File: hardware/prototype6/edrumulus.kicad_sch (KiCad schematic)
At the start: 108 parts, among them J1 Trigger Connector, J2 Raspberry Pi GPIO pins, U1 ESP32-WROOM-32U, U2 AMS1117-3.3, U3 MCP1754S-3302xMB

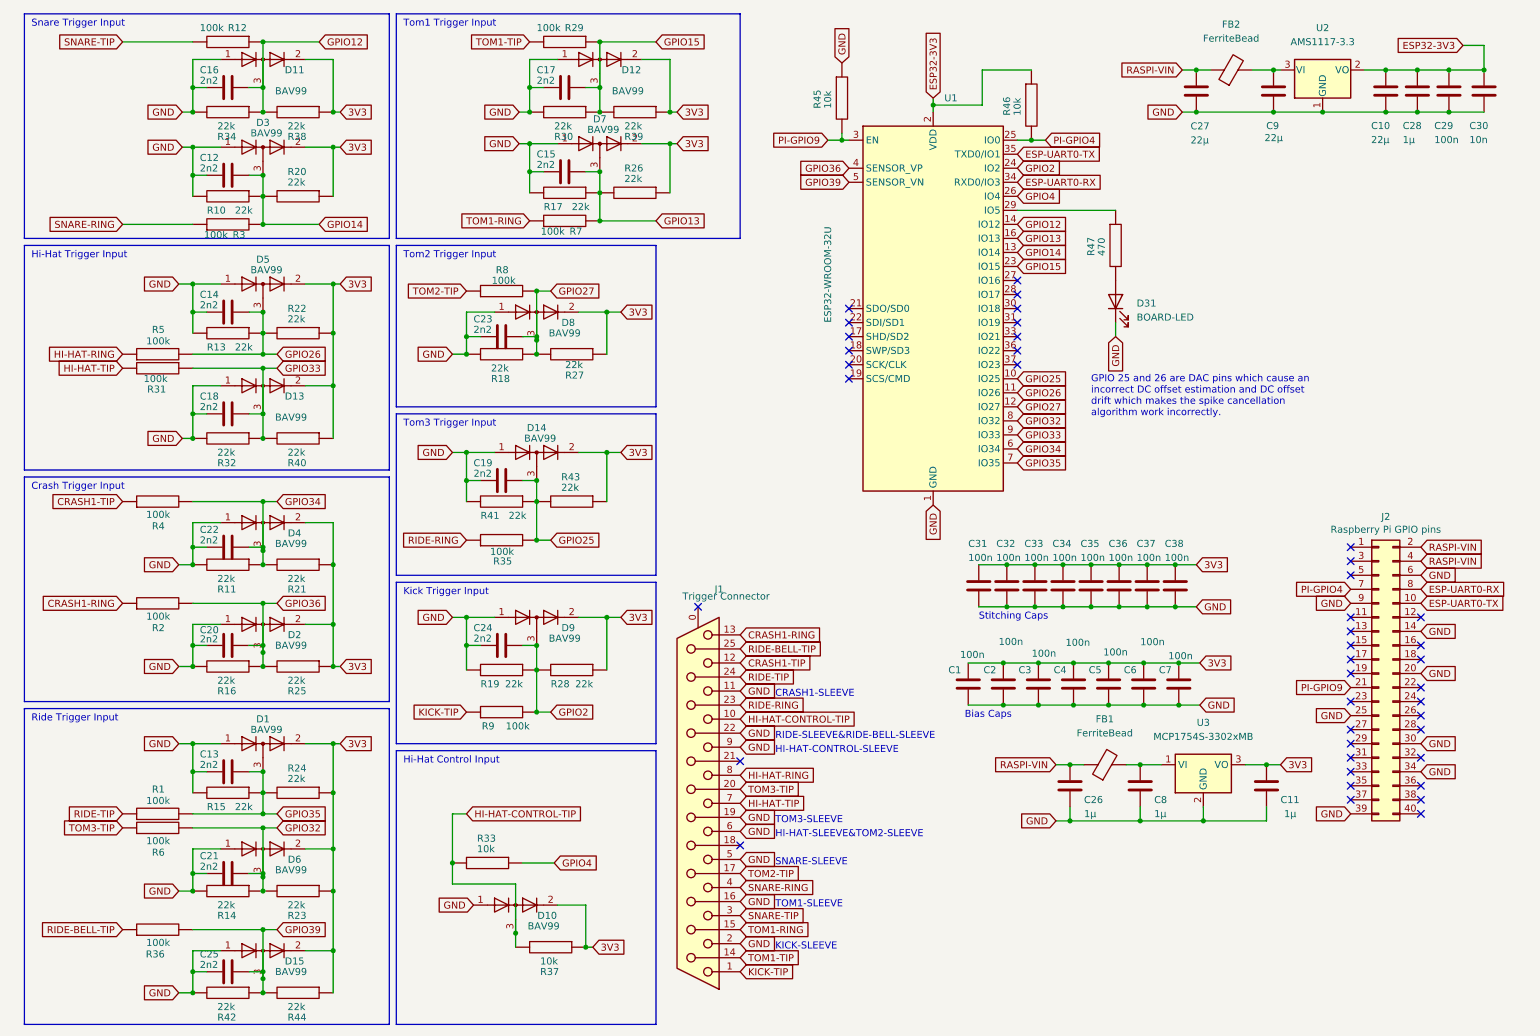
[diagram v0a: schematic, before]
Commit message: some more work on prototpye 6
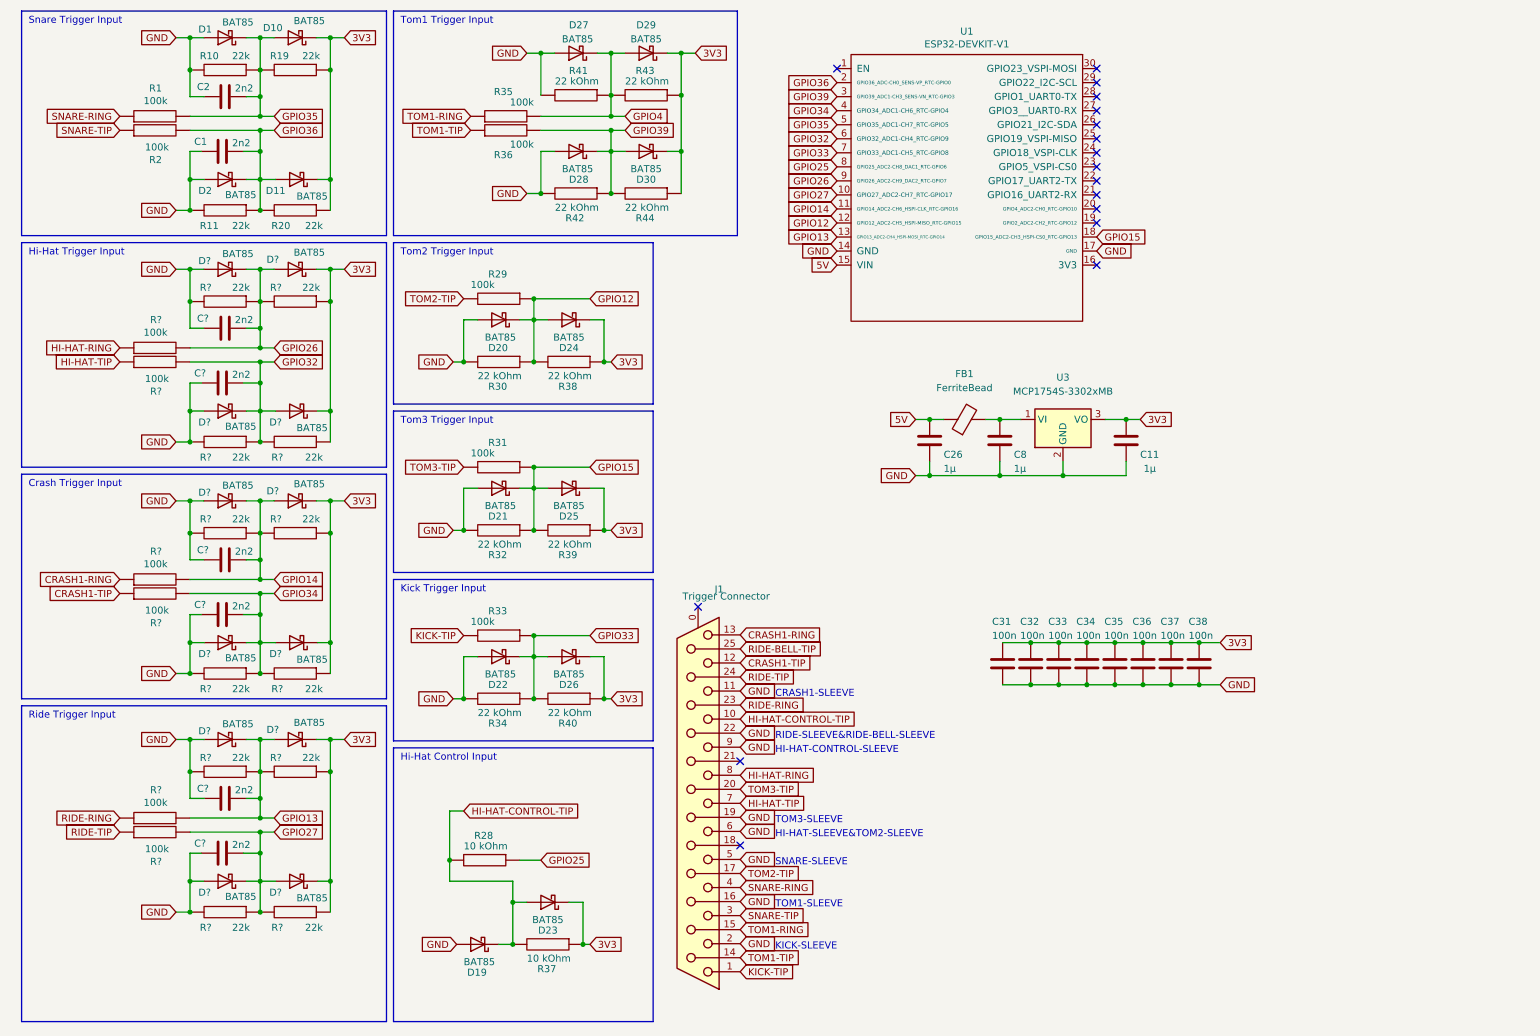
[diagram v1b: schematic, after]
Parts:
- removed C10, C9: 22µ, Capacitor_SMD:C_1210_3225Metric_Pad1.33x2.70mm_HandSolder, symbol Device:C
- removed C12, C13, C14, C15, C16, C17, C18, C19, C20, C21, C22, C23, C24, C25: 2n2, Capacitor_SMD:C_0603_1608Metric_Pad1.08x0.95mm_HandSolder, symbol Device:C
- removed C27: 22µ, Capacitor_SMD:C_0603_1608Metric_Pad1.08x0.95mm_HandSolder, symbol Device:C
- removed C28: 1µ, Capacitor_SMD:C_0603_1608Metric_Pad1.08x0.95mm_HandSolder, symbol Device:C
- removed C29, C3, C4, C5, C6, C7: 100n, Capacitor_SMD:C_0603_1608Metric_Pad1.08x0.95mm_HandSolder, symbol Device:C
- removed C30: 10n, Capacitor_SMD:C_0603_1608Metric_Pad1.08x0.95mm_HandSolder, symbol Device:C
- removed D1, D10, D11, D12, D13, D14, D15, D2, D3, D4, D5, D6, D7, D8, D9: BAV99, Package_TO_SOT_SMD:SOT-23, symbol Diode:BAV99
- removed D31: BOARD-LED, LED_SMD:LED_0603_1608Metric, symbol Device:LED
- removed FB2: FerriteBead, Inductor_SMD:L_1210_3225Metric_Pad1.42x2.65mm_HandSolder, symbol Device:FerriteBead
- removed J2: Raspberry Pi GPIO pins, Connector_PinSocket_2.54mm:PinSocket_2x20_P2.54mm_Vertical, symbol Connector_Generic:Conn_02x20_Odd_Even
- removed R12, R3, R4, R5, R6, R7, R8, R9: 100k, Resistor_SMD:R_0603_1608Metric_Pad0.98x0.95mm_HandSolder, symbol pspice:R
- removed R13, R14, R15, R16, R17, R18, R21, R22, R23, R24, R25, R26, R27: 22k, Resistor_SMD:R_0603_1608Metric_Pad0.98x0.95mm_HandSolder, symbol pspice:R
- removed R45, R46: 10k, Resistor_SMD:R_0603_1608Metric_Pad0.98x0.95mm_HandSolder, symbol pspice:R
- removed R47: 470, Resistor_SMD:R_0603_1608Metric_Pad0.98x0.95mm_HandSolder, symbol pspice:R
- removed U1: ESP32-WROOM-32U, RF_Module:ESP32-WROOM-32U, symbol RF_Module:ESP32-WROOM-32U
- removed U2: AMS1117-3.3, Package_TO_SOT_SMD:SOT-223-3_TabPin2, symbol Regulator_Linear:AMS1117-3.3
- added C? (x6): 2n2, Capacitor_SMD:C_0603_1608Metric_Pad1.08x0.95mm_HandSolder, symbol Device:C
- added D1, D10, D11, D19, D2, D20, D21, D22, D23, D24, D25, D26, D27, D28, D29, D30, D? (x12): BAT85, Diode_THT:D_DO-35_SOD27_P7.62mm_Horizontal, symbol Diode:BAT85
- added R? (x12): 22k, Resistor_SMD:R_1206_3216Metric_Pad1.30x1.75mm_HandSolder, symbol pspice:R
- added R? (x6): 100k, Resistor_SMD:R_1206_3216Metric_Pad1.30x1.75mm_HandSolder, symbol pspice:R
- added U1: ESP32-DEVKIT-V1, edrumulus:esp32_devkit_v1, symbol doit-esp32-devkit-v1:ESP32-DEVKIT-V1
- C1, C2: value 100n -> 2n2
- C11, C26, C31, C32, C33, C34, C35, C36, C37, C38, C8: footprint Capacitor_SMD:C_0603_1608Metric_Pad1.08x0.95mm_HandSolder -> (none)
- R1, R10, R11, R19, R2, R20, R29, R31, R35, R36: footprint Resistor_SMD:R_0603_1608Metric_Pad0.98x0.95mm_HandSolder -> Resistor_SMD:R_1206_3216Metric_Pad1.30x1.75mm_HandSolder
- R28: value 22k -> 10 kOhm; footprint Resistor_SMD:R_0603_1608Metric_Pad0.98x0.95mm_HandSolder -> Resistor_SMD:R_1206_3216Metric_Pad1.30x1.75mm_HandSolder
- R30, R32, R34, R38, R39, R40, R41, R42, R43, R44: value 22k -> 22 kOhm; footprint Resistor_SMD:R_0603_1608Metric_Pad0.98x0.95mm_HandSolder -> Resistor_SMD:R_1206_3216Metric_Pad1.30x1.75mm_HandSolder
- R33: value 10k -> 100k; footprint Resistor_SMD:R_0603_1608Metric_Pad0.98x0.95mm_HandSolder -> Resistor_SMD:R_1206_3216Metric_Pad1.30x1.75mm_HandSolder
- R37: value 10k -> 10 kOhm; footprint Resistor_SMD:R_0603_1608Metric_Pad0.98x0.95mm_HandSolder -> Resistor_SMD:R_1206_3216Metric_Pad1.30x1.75mm_HandSolder
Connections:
- net 3V3: now also R19.1, D10.1 (K), D11.1 (K), D23.1 (K), D24.1 (K), D25.1 (K), D26.1 (K), D29.1 (K), D30.1 (K), D?.1 (K), D?.1 (K), D?.1 (K), D?.1 (K), D?.1 (K), D?.1 (K), R?.1, R?.1, R?.1, R?.1, R?.1, R?.1; no longer C1.2, C2.2, R28.1
- net CRASH1-RING: now also R?.1; no longer R2.1
- net CRASH1-TIP: now also R?.1
- net GND: now also C1.2, C2.2, C?.2, C?.2, C?.2, C?.2, C?.2, C?.2, D1.2 (A), D19.2 (A), D2.2 (A), D20.2 (A), D21.2 (A), D22.2 (A), D27.2 (A), D28.2 (A), D?.2 (A), D?.2 (A), D?.2 (A), D?.2 (A), D?.2 (A), D?.2 (A), R?.2, R?.2, R?.2, R?.2, R?.2, R?.2, U1.14 (GND), U1.17 (GND); no longer C1.1, C2.1, R19.2
- net GPIO12: now also R29.1, R30.1, D20.1 (K), D24.2 (A), U1.12 (GPIO12_ADC2-CH5_HSPI-MISO_RTC-GPIO15); no longer R34.1
- net GPIO13: now also C?.1, D?.1 (K), D?.2 (A), R?.1, R?.2, R?.2, U1.13 (GPIO13_ADC2-CH4_HSPI-MOSI_RTC-GPIO14)
- net GPIO14: now also C?.1, D?.1 (K), D?.2 (A), R?.1, R?.2, R?.2, U1.11 (GPIO14_ADC2-CH6_HSPI-CLK_RTC-GPIO16); no longer R10.1, R20.2
- net GPIO15: now also R31.1, R32.1, D21.1 (K), D25.2 (A), U1.18 (GPIO15_ADC2-CH3_HSPI-CS0_RTC-GPIO13); no longer R29.1, R30.1
- net GPIO25: now also R28.1, U1.8 (GPIO25_ADC2-CH8_DAC1_RTC-GPIO6); no longer R35.2, R41.1, R43.2
- net GPIO26: now also C?.1, D?.1 (K), D?.2 (A), R?.1, R?.2, R?.2, U1.9 (GPIO26_ADC2-CH9_DAC2_RTC-GPIO7)
- net GPIO27: now also C?.1, D?.1 (K), D?.2 (A), R?.1, R?.2, R?.2, U1.10 (GPIO27_ADC2-CH7_RTC-GPIO17)
- net GPIO32: now also C?.1, D?.1 (K), D?.2 (A), R?.1, R?.2, R?.2, U1.6 (GPIO32_ADC1-CH4_RTC-GPIO9)
- net GPIO33: now also R33.1, R34.1, D22.1 (K), D26.2 (A), U1.7 (GPIO33_ADC1-CH5_RTC-GPIO8); no longer R31.1, R32.1
- net GPIO34: now also C?.1, D?.1 (K), D?.2 (A), R?.1, R?.2, R?.2, U1.4 (GPIO34_ADC1-CH6_RTC-GPIO4); no longer R11.1
- net GPIO35: now also C2.1, R10.1, R19.2, D1.1 (K), D10.2 (A), U1.5 (GPIO35_ADC1-CH7_RTC-GPIO5)
- net GPIO36: now also C1.1, R11.1, R20.2, D11.2 (A), D2.1 (K), U1.2 (GPIO36_ADC-CH0_SENS-VP_RTC-GPIO0)
- net GPIO39: now also D28.1 (K), D30.2 (A), U1.3 (GPIO39_ADC1-CH3_SENS-VN_RTC-GPIO3)
- net GPIO4: now also R35.2, R41.1, R43.2, D27.1 (K), D29.2 (A); no longer R33.1
- net HI-HAT-CONTROL-TIP: now also R28.2, D19.1 (K), D23.2 (A); no longer R33.2
- net HI-HAT-RING: now also R?.1
- net HI-HAT-TIP: now also R?.1; no longer R31.2
- net KICK-TIP: now also R33.2
- net RIDE-BELL-TIP: no longer R36.1
- net RIDE-RING: now also R?.1; no longer R35.1
- net RIDE-TIP: now also R?.1; no longer R1.1
- net SNARE-RING: now also R1.1
- net SNARE-TIP: now also R2.1
- net TOM1-RING: now also R35.1
- net TOM1-TIP: now also R36.1; no longer R29.2
- net TOM2-TIP: now also R29.2
- net TOM3-TIP: now also R31.2
- removed net GPIO2: R19.1, R28.2
- net RASPI-VIN renamed 5V
- net 5V: now also U1.15 (VIN)
- no-connect marks 42 -> 17
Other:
- note removed: "Bias Caps"
- note removed: "GPIO 25 and 26 are DAC pins which cause an incorrect DC offset estimation and DC offset drift which makes the spike cancellation algorithm work incorrectly."
- note removed: "Stitching Caps"
- moved on the sheet: C11, C26, C31, C32, C33, C34, C35, C36, C37, C38, C8, FB1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
